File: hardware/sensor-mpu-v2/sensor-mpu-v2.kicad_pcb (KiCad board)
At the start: 2 copper layers, 10 x 40 mm, 24 parts, among them J1 JST SH1.0, Q1 BSS138, Q2 BSS138, U1 LN1134A182MR-G, U2 MPU-9250, U3 MAX30102

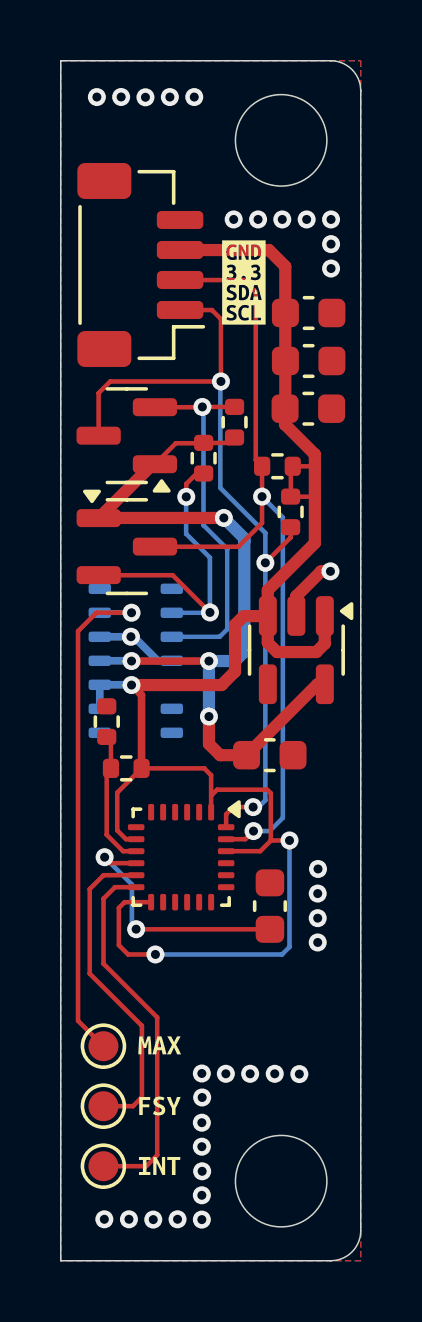
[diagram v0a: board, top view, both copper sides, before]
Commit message: Update for poduction
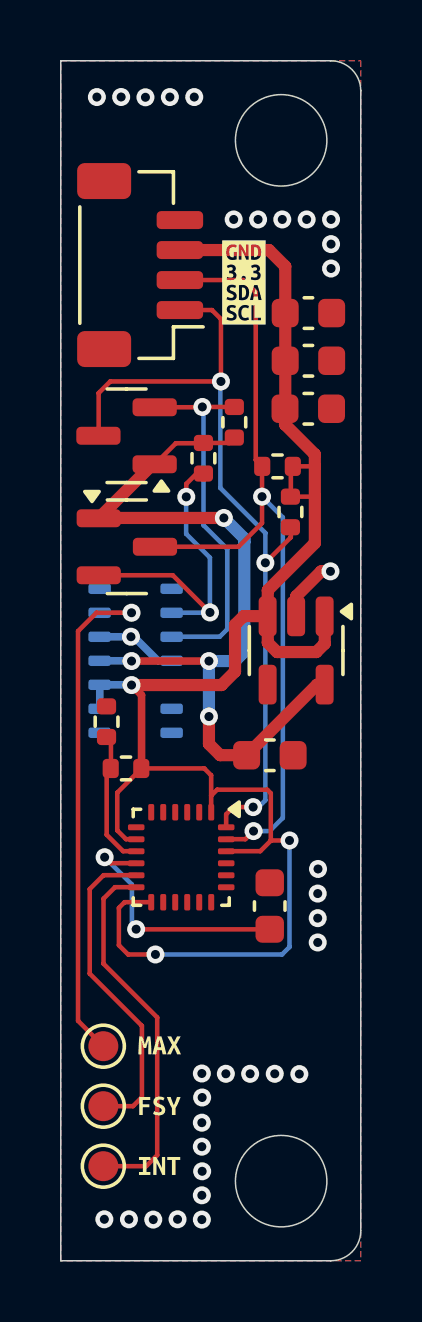
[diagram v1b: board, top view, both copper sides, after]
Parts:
- removed C1: 1uF 16V, Capacitor_SMD:C_0603_1608Metric
- removed C2: 10nF 16V, Capacitor_SMD:C_0603_1608Metric
- removed C3: 2.2uF 16V, Capacitor_SMD:C_0603_1608Metric
- removed C4, C5: 100nF 16V, Capacitor_SMD:C_0603_1608Metric
- removed J1: JST SH1.0, Connector_JST:JST_SH_BM04B-SRSS-TB_1x04-1MP_P1.00mm_Vertical
- removed Q1, Q2: BSS138, Package_TO_SOT_SMD:SOT-23
- removed R1: 0R, Resistor_SMD:R_0402_1005Metric
- removed R2, R3, R4, R5, R6: 10K, Resistor_SMD:R_0402_1005Metric
- removed TP1: MPU_FSYNC, TestPoint:TestPoint_Pad_D1.0mm
- removed TP2: MPU_INT, TestPoint:TestPoint_Pad_D1.0mm
- removed TP3: MAX_INT, TestPoint:TestPoint_Pad_D1.0mm
- removed U1: LN1134A182MR-G, Package_TO_SOT_SMD:SOT-23-5
- removed U2: MPU-9250, Sensor_Motion:InvenSense_QFN-24_3x3mm_P0.4mm_NoMask
- removed U3: MAX30102, OptoDevice:Maxim_OLGA-14_3.3x5.6mm_P0.8mm
- added C81: 1uF 16V, Capacitor_SMD:C_0603_1608Metric, F.Cu at (187.6, 51.6)
- added C82: 10nF 10V, Capacitor_SMD:C_0603_1608Metric, F.Cu at (187.6, 53.2)
- added C83: 2.2uF 16V, Capacitor_SMD:C_0603_1608Metric, F.Cu at (186.3, 66.4)
- added C84: 100nF 10V, Capacitor_SMD:C_0603_1608Metric, F.Cu at (187.6, 54.8)
- added C85: 100nF 10V, Capacitor_SMD:C_0603_1608Metric, F.Cu at (186.3, 71.4)
- added J81: JST SH1.0, Connector_JST:JST_SH_BM04B-SRSS-TB_1x04-1MP_P1.00mm_Vertical, F.Cu at (182.0, 50.0)
- added Q81: BSS138, Package_TO_SOT_SMD:SOT-23, F.Cu at (181.5, 59.4)
- added Q82: BSS138, Package_TO_SOT_SMD:SOT-23, F.Cu at (181.5, 55.7)
- added R81: DNP, Resistor_SMD:R_0402_1005Metric, F.Cu at (181.5, 66.8)
- added R82: 10K, Resistor_SMD:R_0402_1005Metric, F.Cu at (180.8, 65.2)
- added R83: 10K, Resistor_SMD:R_0402_1005Metric, F.Cu at (185.1, 55.3)
- added R84: 10K, Resistor_SMD:R_0402_1005Metric, F.Cu at (184.1, 56.5)
- added R85: 10K, Resistor_SMD:R_0402_1005Metric, F.Cu at (187.0, 58.2)
- added R86: 10K, Resistor_SMD:R_0402_1005Metric, F.Cu at (186.5, 56.7)
- added TP81: MPU_FSYNC, TestPoint:TestPoint_Pad_D1.0mm, F.Cu at (180.7, 78.1)
- added TP82: MPU_INT, TestPoint:TestPoint_Pad_D1.0mm, F.Cu at (180.7, 80.1)
- added TP83: MAX_INT, TestPoint:TestPoint_Pad_D1.0mm, F.Cu at (180.7, 76.1)
- added U81: LN1134A182MR-G, Package_TO_SOT_SMD:SOT-23-5, F.Cu at (187.2, 62.9)
- added U82: MPU-9250, Sensor_Motion:InvenSense_QFN-24_3x3mm_P0.4mm_NoMask, F.Cu at (183.3, 69.8)
- added U83: MAX30102, OptoDevice:Maxim_OLGA-14_3.3x5.6mm_P0.8mm, B.Cu at (181.8, 63.2)
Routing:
- net Net-(U83-~{INT}): track 0.00 -> 17.3 mm, vias 0 -> 1
- net Net-(U3-~{INT}): track 17.3 -> 0.00 mm, vias 1 -> 0
- net Net-(U82-INT): track 0.00 -> 12.5 mm
- net Net-(U2-INT): track 12.5 -> 0.00 mm
- net Net-(U82-FSYNC): track 0.00 -> 10.8 mm
- net Net-(U2-FSYNC): track 10.8 -> 0.00 mm
- net Net-(U82-REGOUT): track 0.00 -> 8.43 mm, vias 0 -> 2
- net Net-(U2-REGOUT): track 8.43 -> 0.00 mm, vias 2 -> 0
- net Net-(U82-AD0/MISO): track 0.00 -> 4.59 mm
- net Net-(U2-AD0/MISO): track 4.59 -> 0.00 mm
